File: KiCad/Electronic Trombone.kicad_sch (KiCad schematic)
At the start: 3 parts, among them J1 691137710002

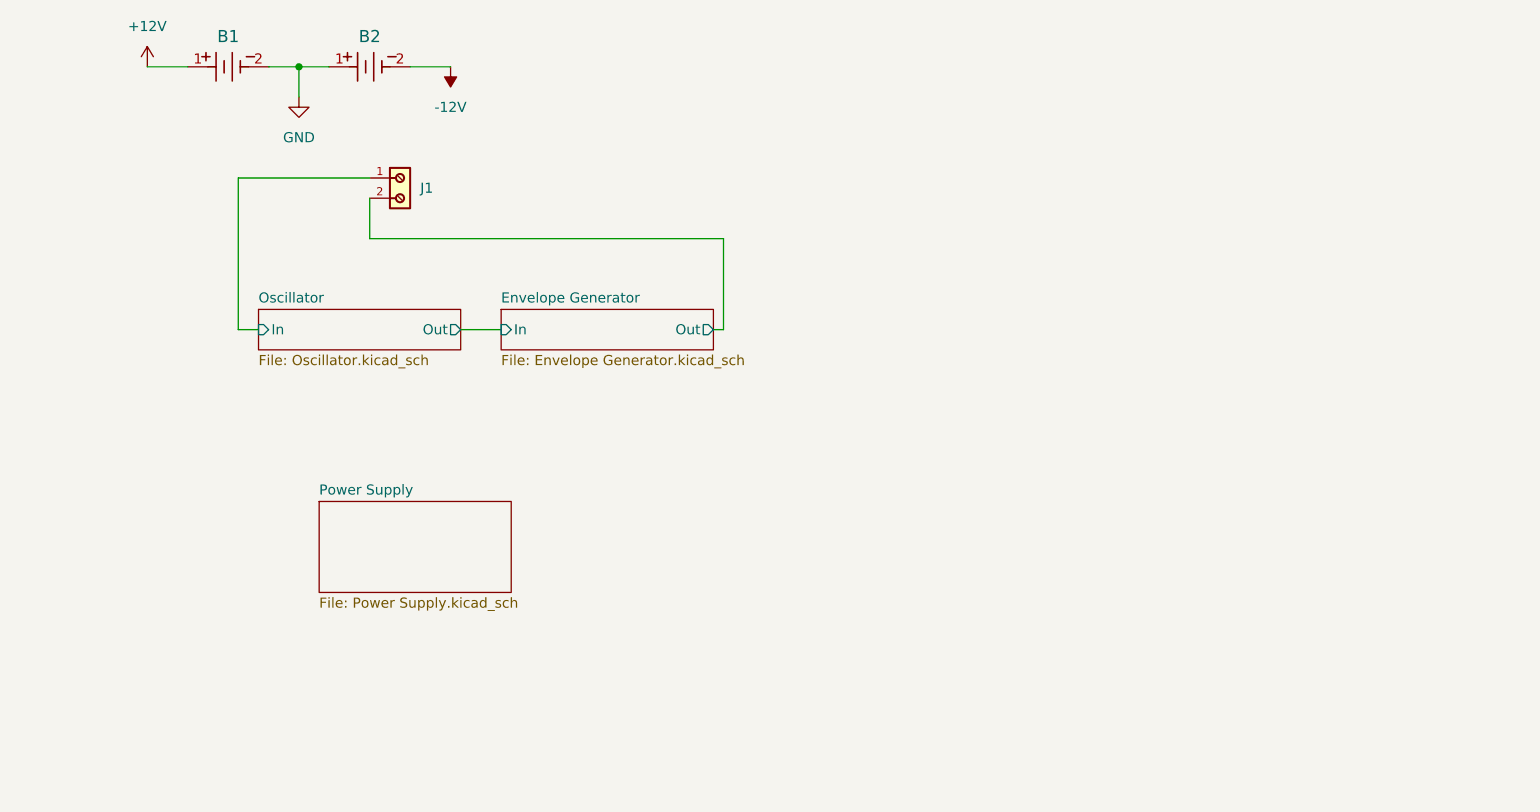
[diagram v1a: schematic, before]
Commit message: amplifier sch., general changes to oscillator sch.
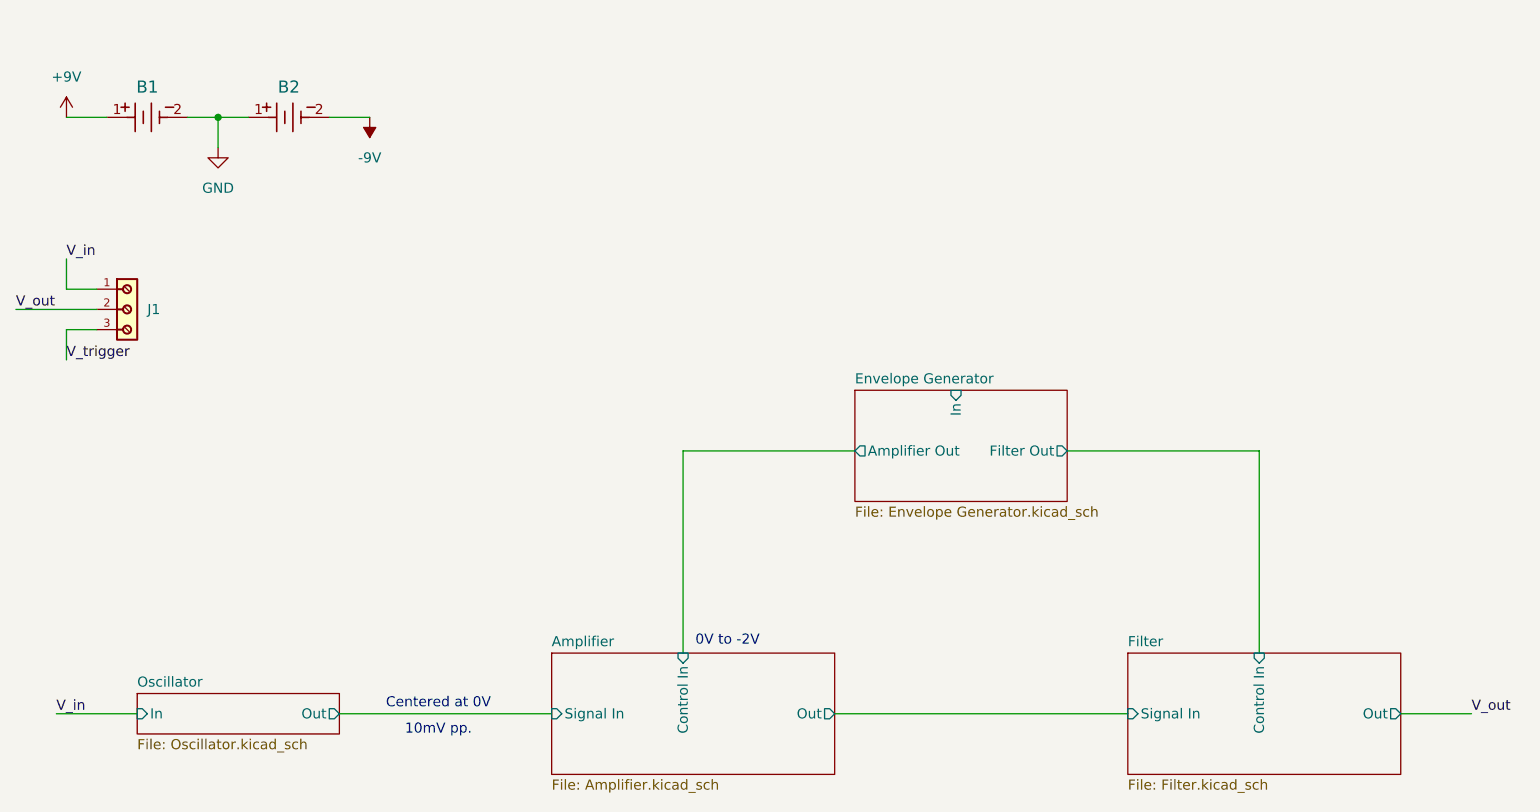
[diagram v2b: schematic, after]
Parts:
- removed J1: 691137710002, Header 691137710002:691137710002, symbol 691137710002:691137710002
- added J1: 691137710003, 691137710003:691137710003, symbol Header 691137710003:691137710003
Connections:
- net +12V renamed +9V
- net -12V renamed -9V
- new net V_in: J1.1
- new net V_out: J1.2
- new net V_trigger: J1.3
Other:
- removed sheet Power Supply
- added sheet Amplifier (Amplifier.kicad_sch)
- added sheet Filter (Filter.kicad_sch)
- sheet Envelope Generator ports: added Amplifier Out, Filter Out; removed Out
- note added: "0V to -2V"
- note added: "10mV pp."
- note added: "Centered at 0V"
- moved on the sheet: B1, B2
